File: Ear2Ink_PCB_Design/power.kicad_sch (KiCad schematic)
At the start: 1 part, among them U2 TPS562208DDCR

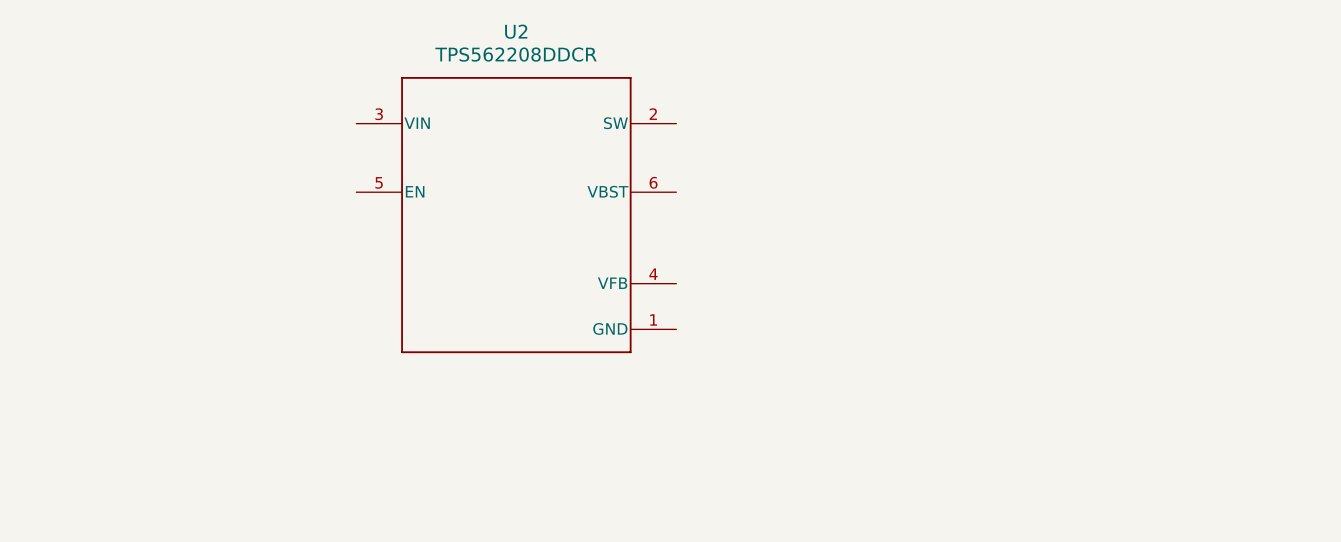
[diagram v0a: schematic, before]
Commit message: added buck
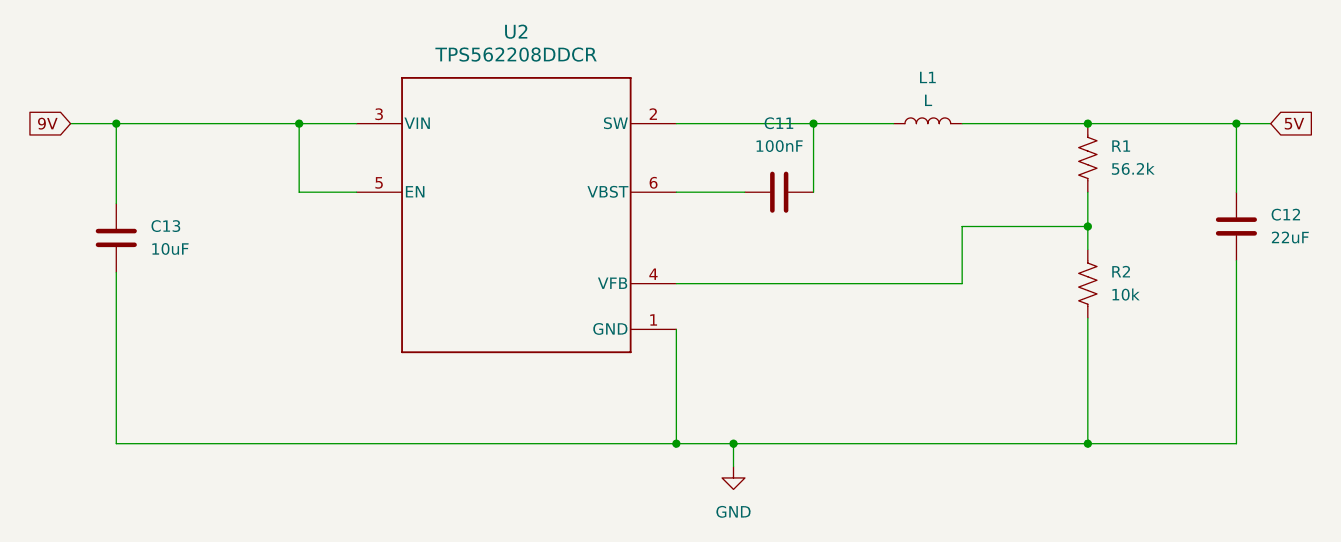
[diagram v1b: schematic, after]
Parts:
- added C11: 100nF, symbol Device:C
- added C12: 22uF, symbol Device:C
- added C13: 10uF, symbol Device:C
- added L1: L, symbol Device:L
- added R1: 56.2k, symbol Device:R_US
- added R2: 10k, symbol Device:R_US
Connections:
- net GND: now reaches U2.1 (GND)
- net GND: now also C12.2, C13.1, R2.2
- net at U2.2 (SW): now also C11.2, L1.1
- net 9V: now reaches U2.3 (VIN)
- net 9V: now also U2.5 (EN), C13.2
- net at U2.4 (VFB): now also R1.2, R2.1
- net at U2.6 (VBST): now also C11.1
- new net 5V: C12.1, L1.2, R1.1
